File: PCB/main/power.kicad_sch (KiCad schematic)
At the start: 38 parts, among them IC1 TP4056-42-ESOP8, IC2 AMS1117-3.3, J5 Conn_01x33_Female, J6 Conn_01x33_Female, J7 MICROXNJ, Q1 Q_PNP_BCE, Q2 Q_NMOS_DSG, Q3 BC857, Q4 Q_PMOS_GDS, Q5 2N3904, U1 LM393

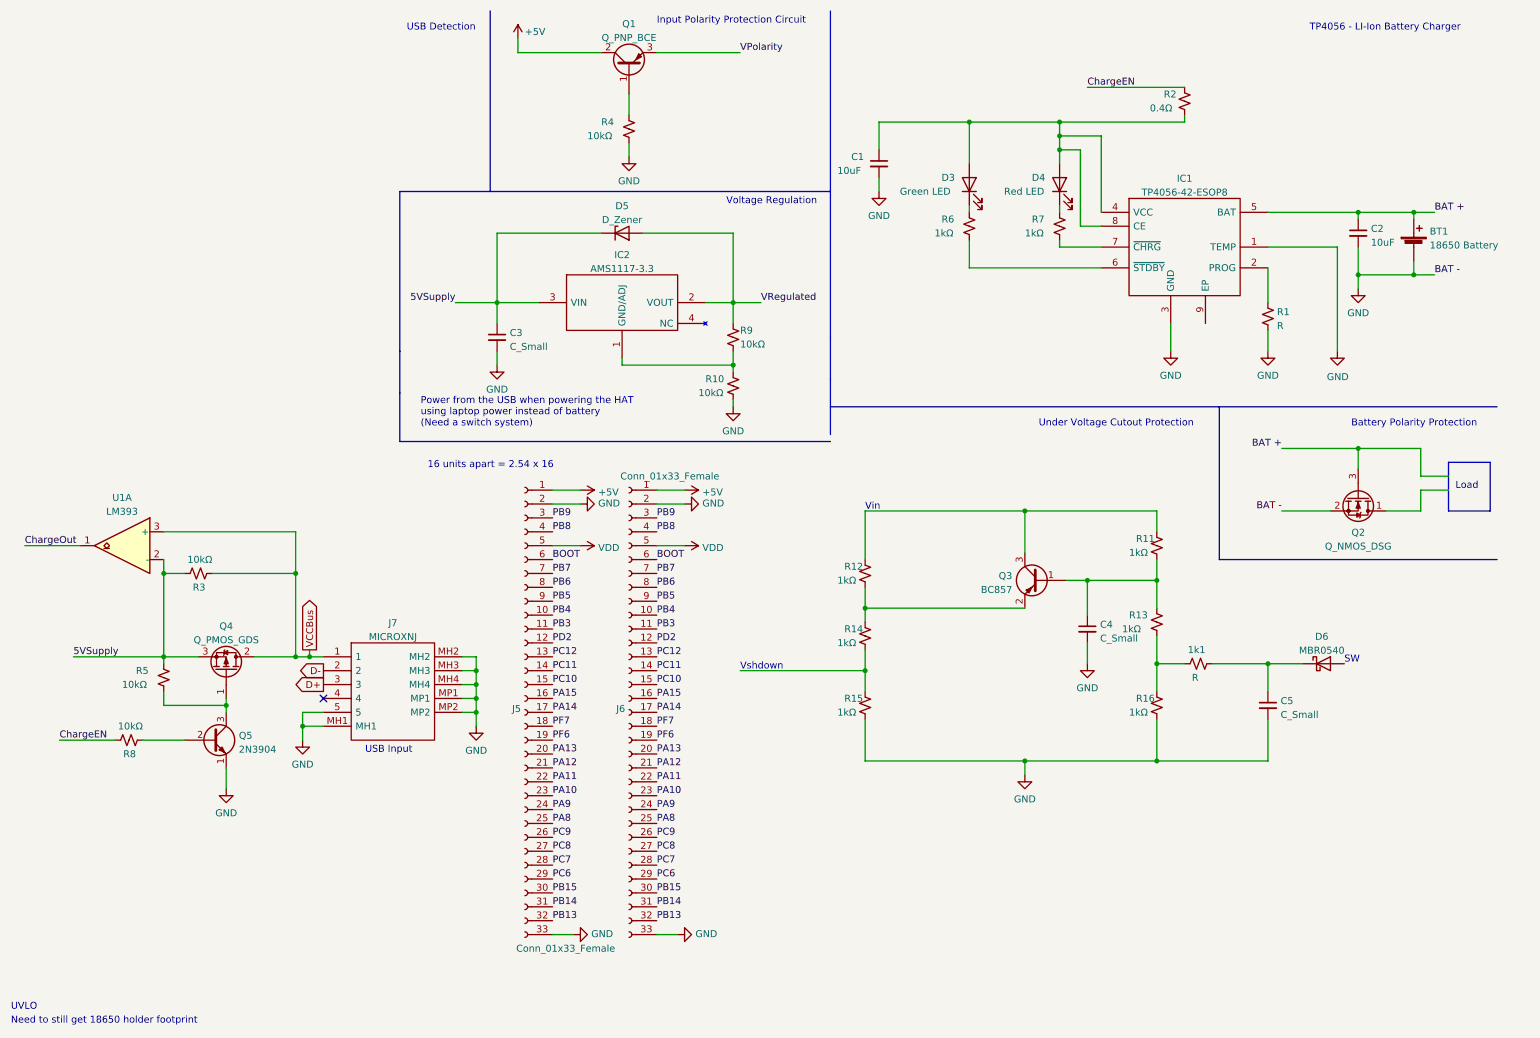
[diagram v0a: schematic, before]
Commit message: Power Module v0.03
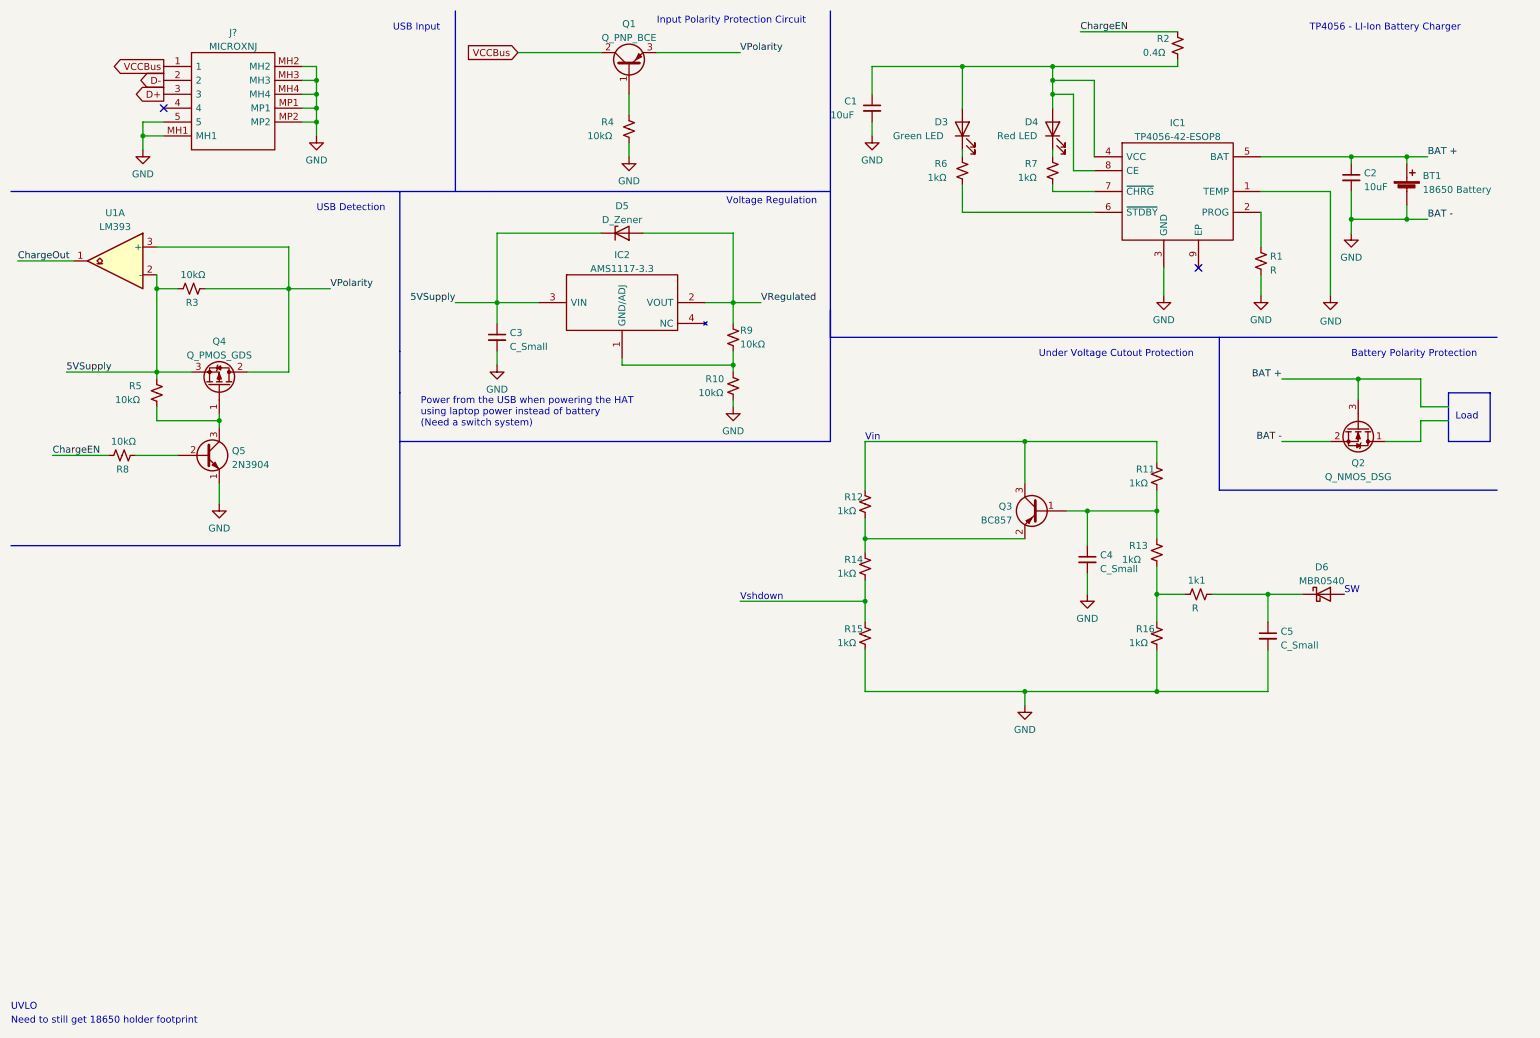
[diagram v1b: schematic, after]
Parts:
- removed J5: Conn_01x33_Female, Connector_PinSocket_2.54mm:PinSocket_1x33_P2.54mm_Vertical, symbol Connector:Conn_01x33_Female
- removed J6: Conn_01x33_Female, Connector_PinHeader_2.54mm:PinHeader_1x33_P2.54mm_Vertical, symbol Connector:Conn_01x33_Female
- removed J7: MICROXNJ, MICROXNJ, symbol MICROXNJ:MICROXNJ
- added J?: MICROXNJ, MICROXNJ, symbol MICROXNJ:MICROXNJ
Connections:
- net +5V is gone; now on net VCCBus: Q1.2 (C)
- net D+: now also J?.3
- net D-: now also J?.2
- net GND: now also J?.5, J?.MH1, J?.MH2, J?.MH3, J?.MH4, J?.MP1, J?.MP2
- net VCCBus: now also J?.1; no longer Q4.2 (D), R3.2, U1.3 (+)
- net VPolarity: now also Q4.2 (D), R3.2, U1.3 (+)
- no-connect marks 1 -> 2
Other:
- note removed: "16 units apart = 2.54 x 16"
- moved on the sheet: 1k1, BT1, C1, C2, C4, C5, D3, D4, D6, IC1, Q2, Q3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
